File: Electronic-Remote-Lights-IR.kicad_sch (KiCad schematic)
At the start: 17 parts, among them J1 POWER_PINS, J2 POWER_USB, J3 RELAY, SW1 RESET, U1 VS1338B

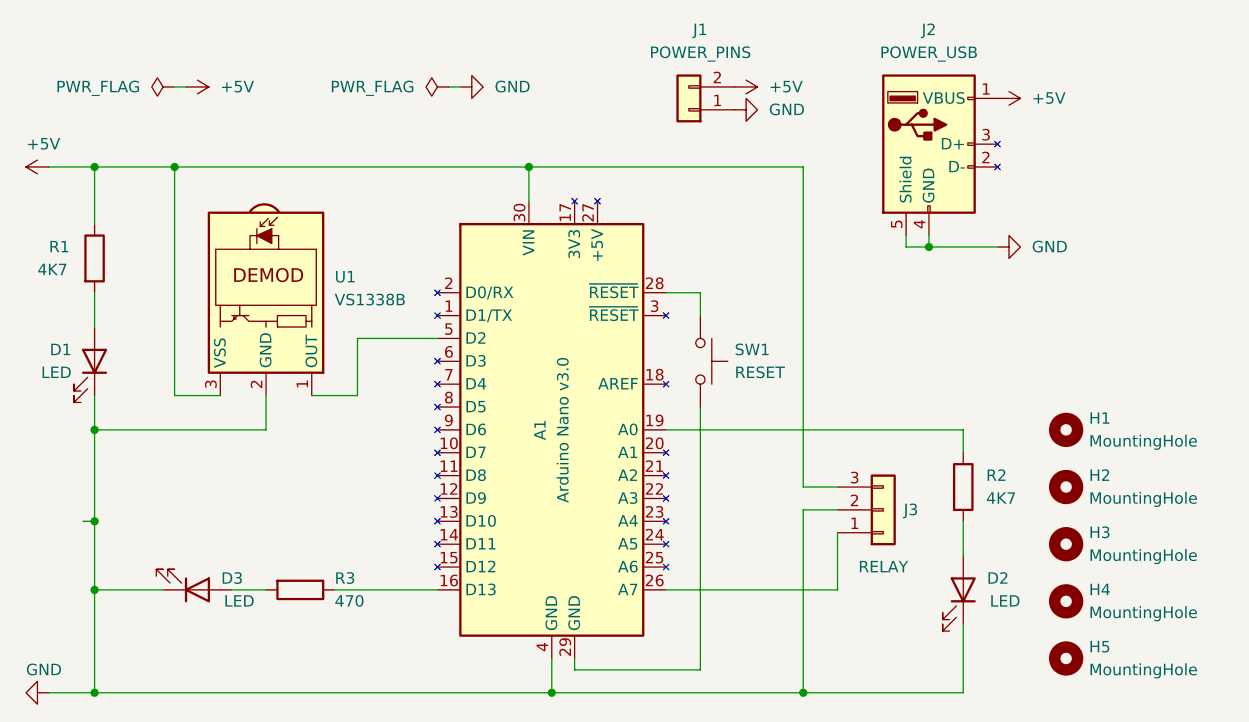
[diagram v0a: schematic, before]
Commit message: rearrange assigned pins
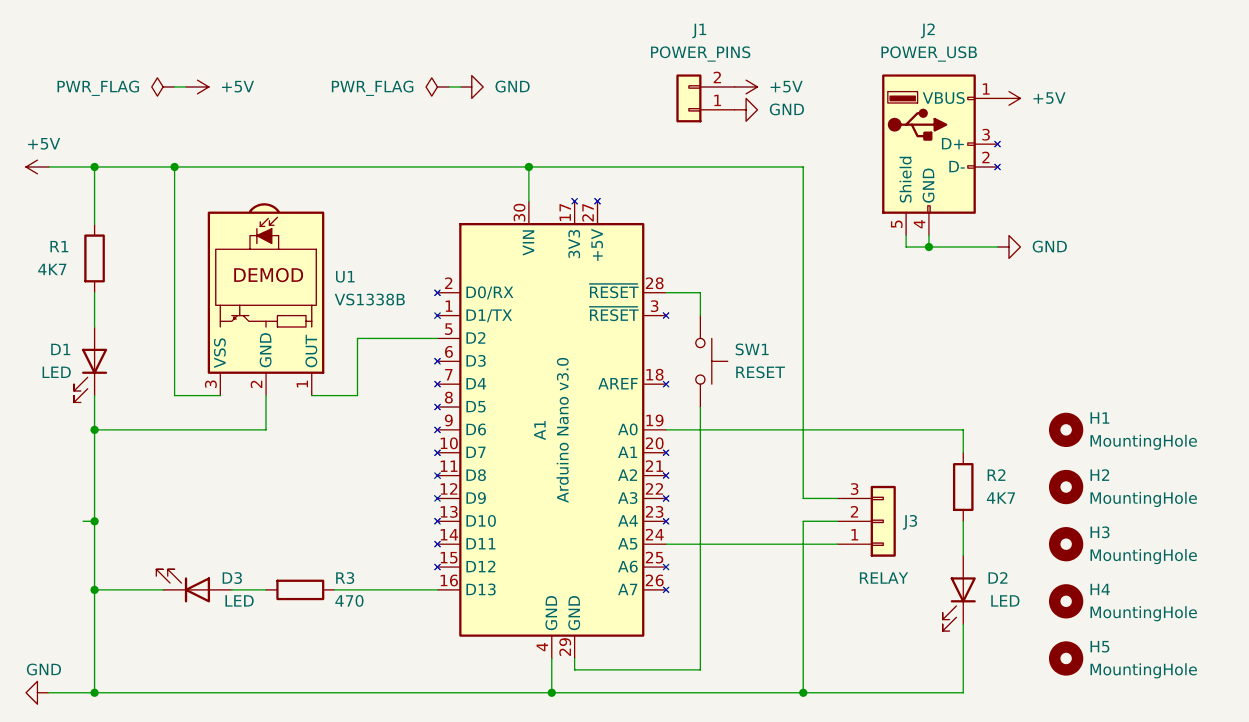
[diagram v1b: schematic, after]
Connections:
- net at A1.24 (A5): now also J3.1 (Pin_1)
- net at A1.26 (A7): no longer J3.1 (Pin_1)
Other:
- moved on the sheet: J3
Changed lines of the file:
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@@
+    (stroke (width 0) (type default) (color 0 0 0 0))
+  )
+  (wire (pts (xy 115.57 121.92) (xy 134.62 121.92))
     (stroke (width 0) (type default) (color 0 0 0 0))
   )
@@
     (stroke (width 0) (type default) (color 0 0 0 0))
   )
-  (wire (pts (xy 130.81 118.11) (xy 130.81 138.43))
-    (stroke (width 0) (type default) (color 0 0 0 0))
-  )
   (wire (pts (xy 46.99 138.43) (xy 52.07 138.43))
     (stroke (width 0) (type default) (color 0 0 0 0))
   )
-  (wire (pts (xy 115.57 127) (xy 134.62 127))
-    (stroke (width 0) (type default) (color 0 0 0 0))
-  )
   (wire (pts (xy 152.4 88.9) (xy 144.78 88.9))
     (stroke (width 0) (type default) (color 0 0 0 0))
@@
     (stroke (width 0) (type default) (color 0 0 0 0))
   )
-  (wire (pts (xy 134.62 118.11) (xy 130.81 118.11))
+  (wire (pts (xy 130.81 119.38) (xy 130.81 138.43))
+    (stroke (width 0) (type default) (color 0 0 0 0))
+  )
+  (wire (pts (xy 134.62 119.38) (xy 130.81 119.38))
     (stroke (width 0) (type default) (color 0 0 0 0))
   )
@@
     (stroke (width 0) (type default) (color 0 0 0 0))
   )
-  (wire (pts (xy 134.62 115.57) (xy 130.81 115.57))
-    (stroke (width 0) (type default) (color 0 0 0 0))
-  )
-  (wire (pts (xy 134.62 120.65) (xy 134.62 127))
+  (wire (pts (xy 134.62 116.84) (xy 130.81 116.84))
     (stroke (width 0) (type default) (color 0 0 0 0))
   )
@@
     (stroke (width 0) (type default) (color 0 0 0 0))
   )
-  (wire (pts (xy 130.81 115.57) (xy 130.81 80.01))
+  (wire (pts (xy 130.81 80.01) (xy 130.81 116.84))
     (stroke (width 0) (type default) (color 0 0 0 0))
   )
@@
     (pin "1")
   )
-  (symbol (lib_id "Connector_Generic:Conn_01x03") (at 139.7 118.11 0) (mirror x) (unit 1)
-    (in_bom yes) (on_board yes)
-    (property "Reference" "J3" (id 0) (at 142.79 118.11 0))
-    (property "Value" "RELAY" (id 1) (at 139.7 124.46 0))
-    (property "Footprint" "Connector_PinHeader_2.54mm:PinHeader_1x03_P2.54mm_Horizontal" (id 2) (at 139.7 118.11 0)
-      (effects (font (size 1.27 1.27)) hide)
-    )
-    (property "Datasheet" "~" (id 3) (at 139.7 118.11 0)
-      (effects (font (size 1.27 1.27)) hide)
-    )
+  (symbol (lib_id "Connector_Generic:Conn_01x03") (at 139.7 119.38 0) (mirror x) (unit 1)
+    (in_bom yes) (on_board yes)
+    (property "Reference" "J3" (id 0) (at 142.79 119.38 0))
+    (property "Value" "RELAY" (id 1) (at 139.7 125.73 0))
+    (property "Footprint" "Connector_PinHeader_2.54mm:PinHeader_1x03_P2.54mm_Horizontal" (id 2) (at 139.7 119.38 0)
+      (effects (font (size 1.27 1.27)) hide)
+    )
+    (property "Datasheet" "~" (id 3) (at 139.7 119.38 0)
+      (effects (font (size 1.27 1.27)) hide)
+    )
